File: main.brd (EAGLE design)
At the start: 50.9 x 36.8 mm, 3 parts

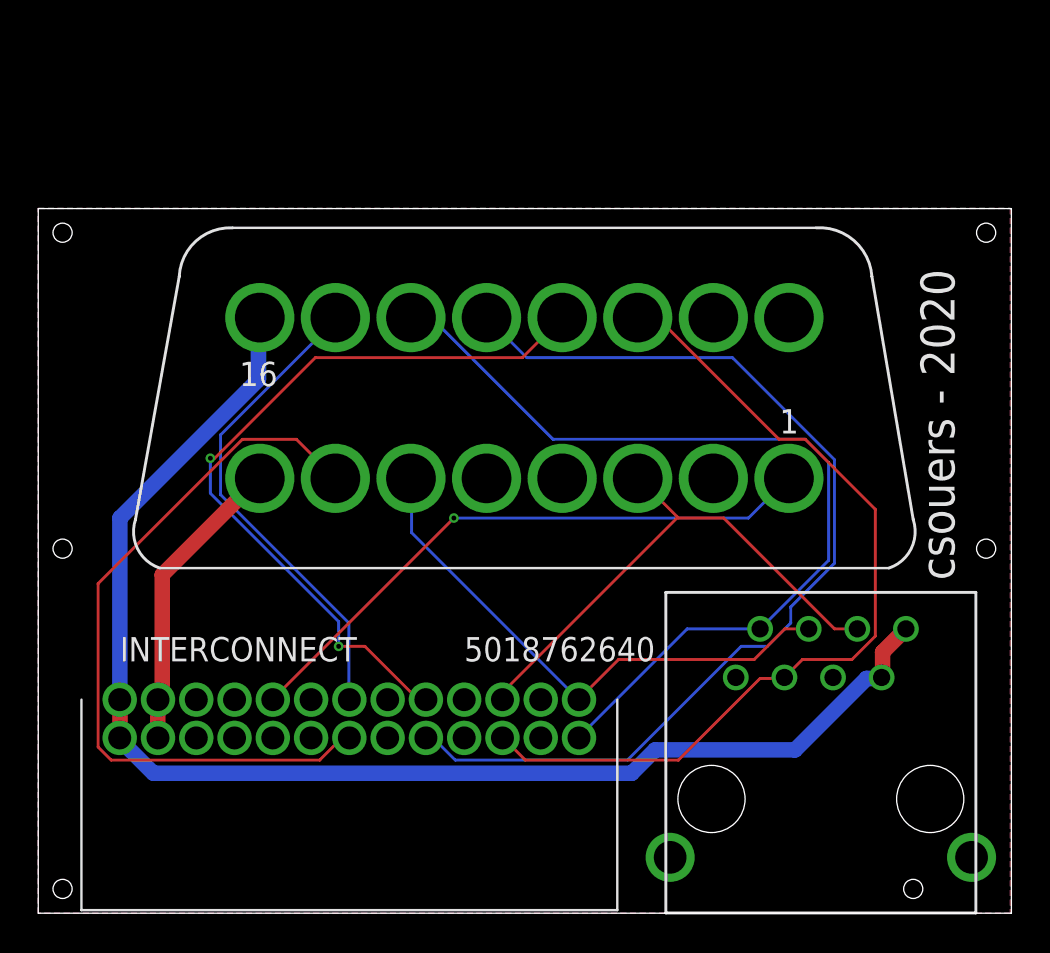
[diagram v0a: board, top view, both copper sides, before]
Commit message: push new versions. autorouted!
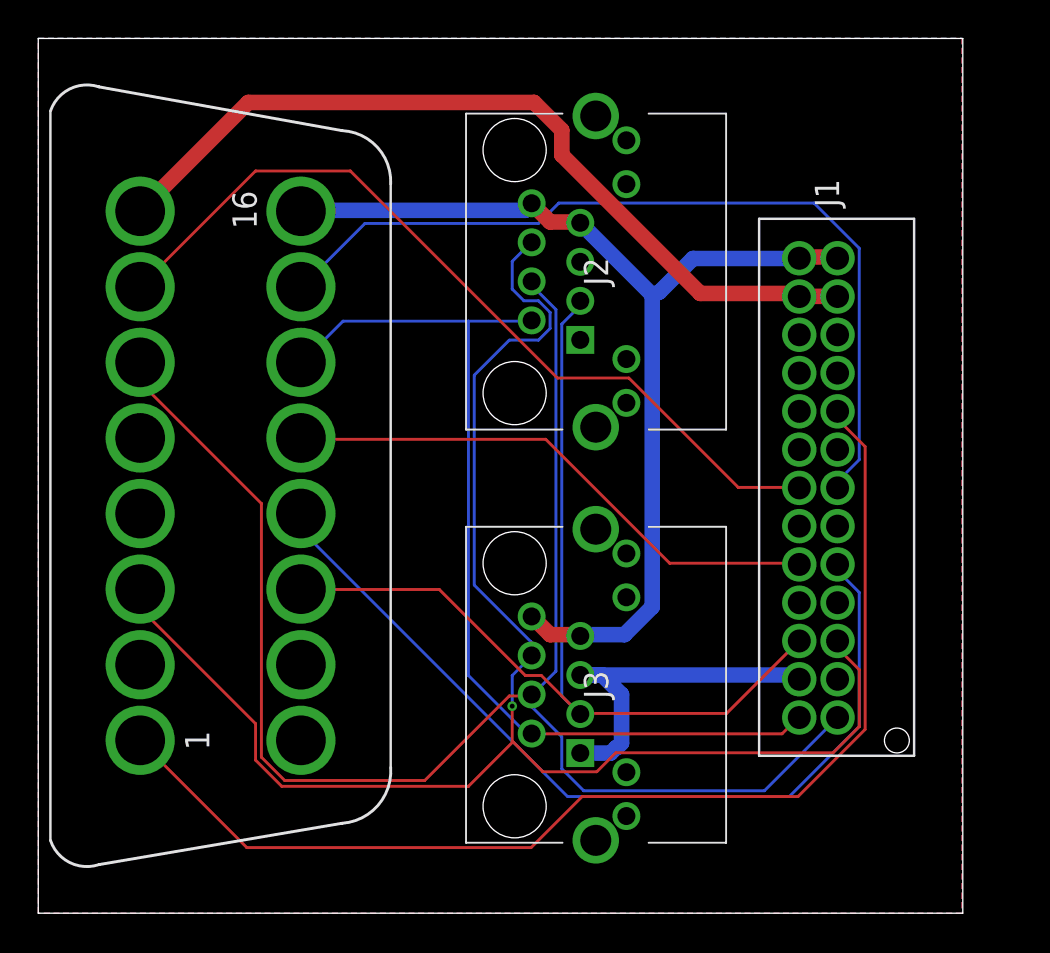
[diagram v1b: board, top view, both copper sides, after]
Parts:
- removed ETHERNET: RA-RJ45RA-2, comma.ai:RA-RJ45-2
- removed INTERCONNECT: 5018762640, Souers:5018762640
- added J1: 501645-2620, Souers:501645-2620
- added J2, J3: RJHSE-3380, RJHSE-3380:RJHSE3384
- moved PANDA 16.4 mm to (9.53, 22.9), turned to 270 degrees
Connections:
- removed net BCAN_H: INTERCONNECT.10, PANDA.12
- removed net BCAN_L: INTERCONNECT.9, PANDA.13
- removed net FCAN_A_H: ETHERNET.4, INTERCONNECT.2, PANDA.6
- removed net FCAN_A_L: ETHERNET.2, INTERCONNECT.1, PANDA.14
- removed net FCAN_B_H: ETHERNET.6, INTERCONNECT.6, PANDA.3
- removed net FCAN_B_L: ETHERNET.3, INTERCONNECT.5, PANDA.11
- new net CAN0_H: J1.2, J2.4, J3.4, PANDA.6
- new net CAN0_L: J1.1, J2.2, J3.2, PANDA.14
- new net CAN1_H: J1.6, J2.6, J3.6, PANDA.3
- new net CAN1_L: J1.5, J2.3, J3.3, PANDA.11
- new net CAN2_H: J1.10, PANDA.12
- new net CAN2_L: J1.9, PANDA.13
- net AUX2: now also J1.17; no longer INTERCONNECT.17
- net AUX3: now also J1.20; no longer INTERCONNECT.20
- net AUX4: now also J1.19; no longer INTERCONNECT.19
- net GMLAN: now also J1.18; no longer INTERCONNECT.18
- net GND: now also J1.11, J1.12, J1.15, J1.16, J1.21, J1.22, J1.3, J1.4, J1.7, J1.8, J2.1, J2.5, J3.1, J3.5; no longer ETHERNET.1, ETHERNET.5, INTERCONNECT.11, INTERCONNECT.12, INTERCONNECT.15, INTERCONNECT.16, INTERCONNECT.21, INTERCONNECT.22, INTERCONNECT.3, INTERCONNECT.4, INTERCONNECT.7, INTERCONNECT.8
- net IGN: now also J1.23, J1.24; no longer INTERCONNECT.23, INTERCONNECT.24
- net K_LINE: now also J1.13; no longer INTERCONNECT.13
- net L_LINE: now also J1.14; no longer INTERCONNECT.14
- net VIN: now also J1.25, J1.26, J2.7, J2.8, J3.7, J3.8; no longer ETHERNET.7, ETHERNET.8, INTERCONNECT.25, INTERCONNECT.26
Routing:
- net CAN0_H: track 0.00 -> 83.4 mm
- net CAN1_H: track 0.00 -> 83.1 mm, vias 0 -> 1
- net BCAN_L: track 53.2 -> 0.00 mm
- net CAN1_L: track 0.00 -> 52.7 mm
- net CAN0_L: track 0.00 -> 50.4 mm
- net FCAN_A_L: track 47.0 -> 0.00 mm
- net CAN2_H: track 0.00 -> 46.3 mm
- net FCAN_B_L: track 45.8 -> 0.00 mm
- net BCAN_H: track 39.7 -> 0.00 mm, vias 2 -> 0
- net CAN2_L: track 0.00 -> 28.8 mm
- net FCAN_A_H: track 28.8 -> 0.00 mm
- net GMLAN: track 31.8 -> 60.0 mm, vias 1 -> 0
- net FCAN_B_H: track 28.1 -> 0.00 mm
- net IGN: track 15.8 -> 43.7 mm
- net L_LINE: track 25.2 -> 45.0 mm
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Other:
- board size 50.9 x 36.8 mm -> 48.3 x 45.7 mm
- board text added: "body harness - main board"
- board text added: "csouers 7/1/2020"
- board text added: "github.com/csouers/bodyharness"
- board text removed: "BCM harness - Main Board"
- board text removed: "csouers - 2020"
- board text removed: "github.com/csouers/bcmharness"
